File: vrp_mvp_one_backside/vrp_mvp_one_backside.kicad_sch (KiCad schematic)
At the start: 7 parts, among them J2 BACKSIDE_INTERFACE, J7 BACKSIDE_INTERFACE_2, Q2 MMBT2222A

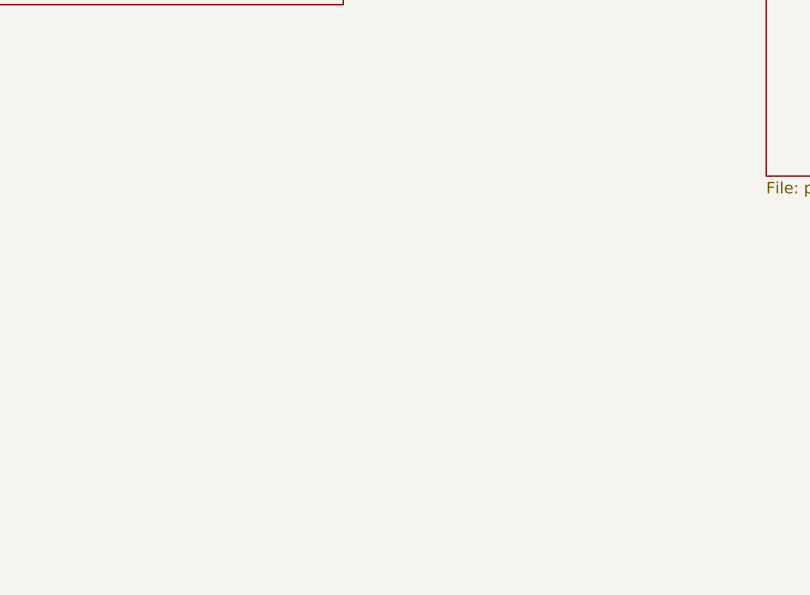
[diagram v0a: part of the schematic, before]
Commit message: minor changes
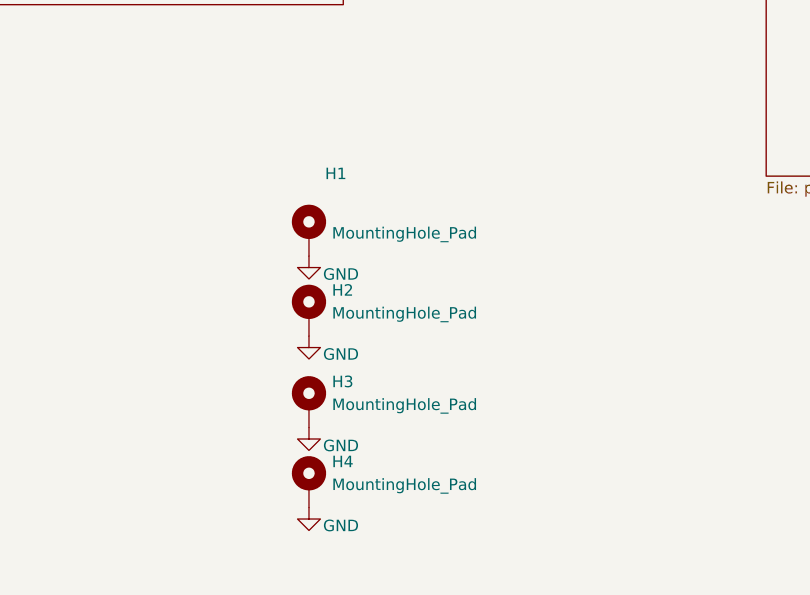
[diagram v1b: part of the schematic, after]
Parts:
- added H1, H2, H3, H4: MountingHole_Pad, MountingHole:MountingHole_2.7mm_M2.5_DIN965_Pad, symbol Mechanical:MountingHole_Pad
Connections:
- net GND: now also H1.1, H2.1, H3.1, H4.1
